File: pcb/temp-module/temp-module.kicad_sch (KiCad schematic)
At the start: 12 parts, among them J1 Connector_male, J2 Screw_Terminal_01x02, U1 MCP6002-xSN

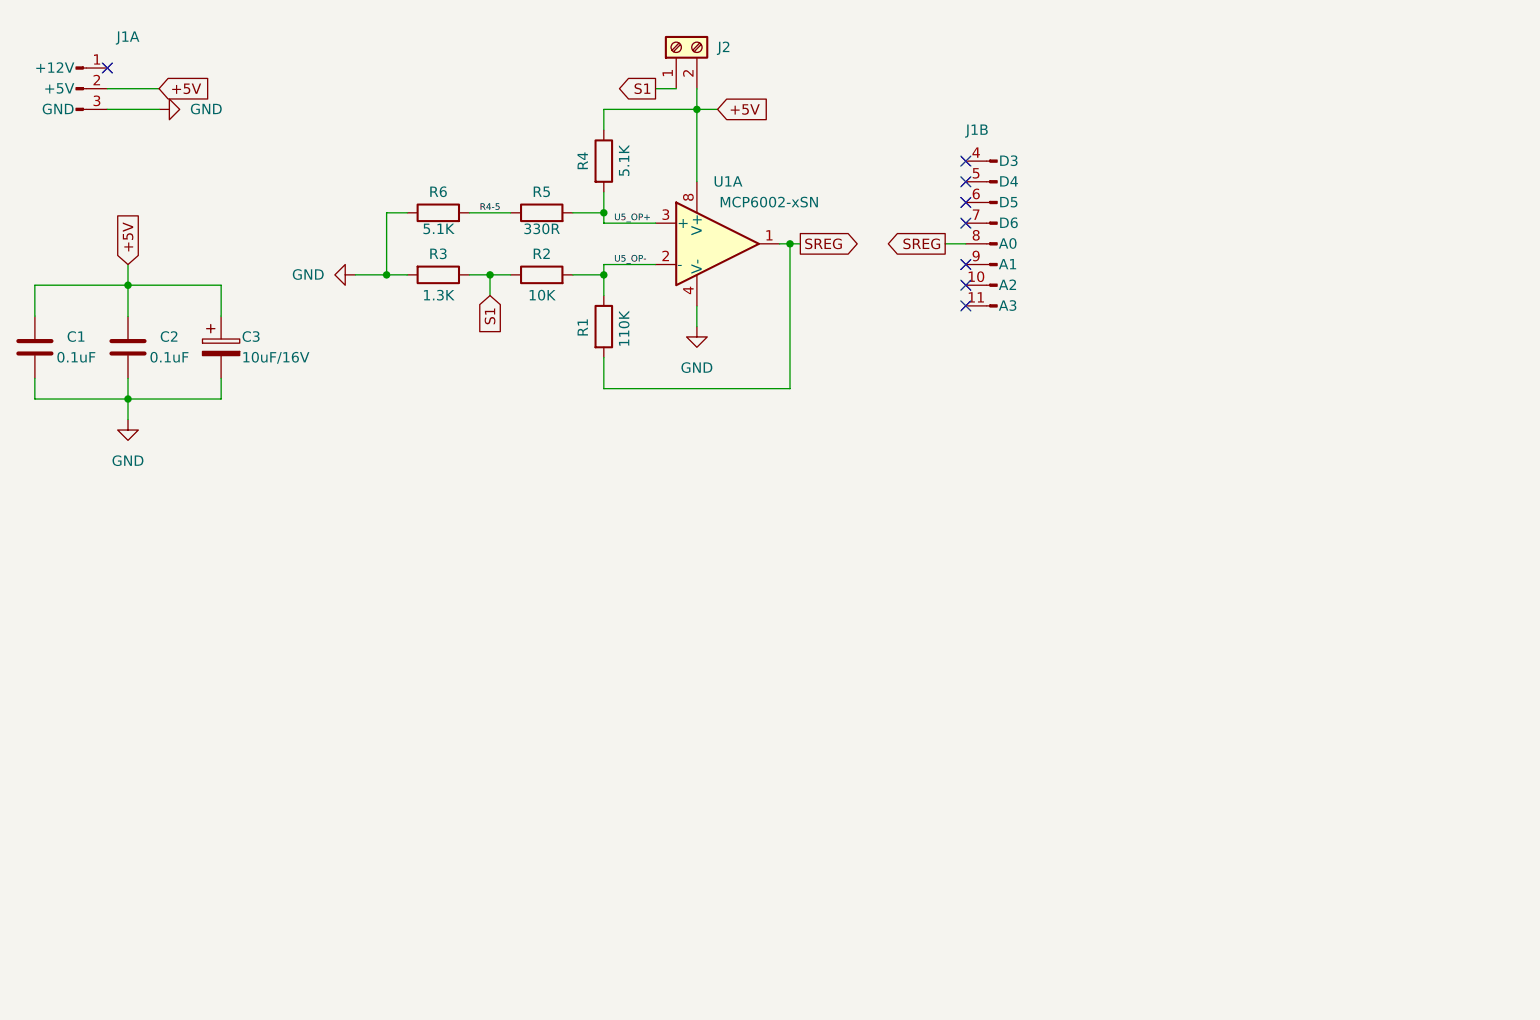
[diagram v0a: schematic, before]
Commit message: temp-calibrate
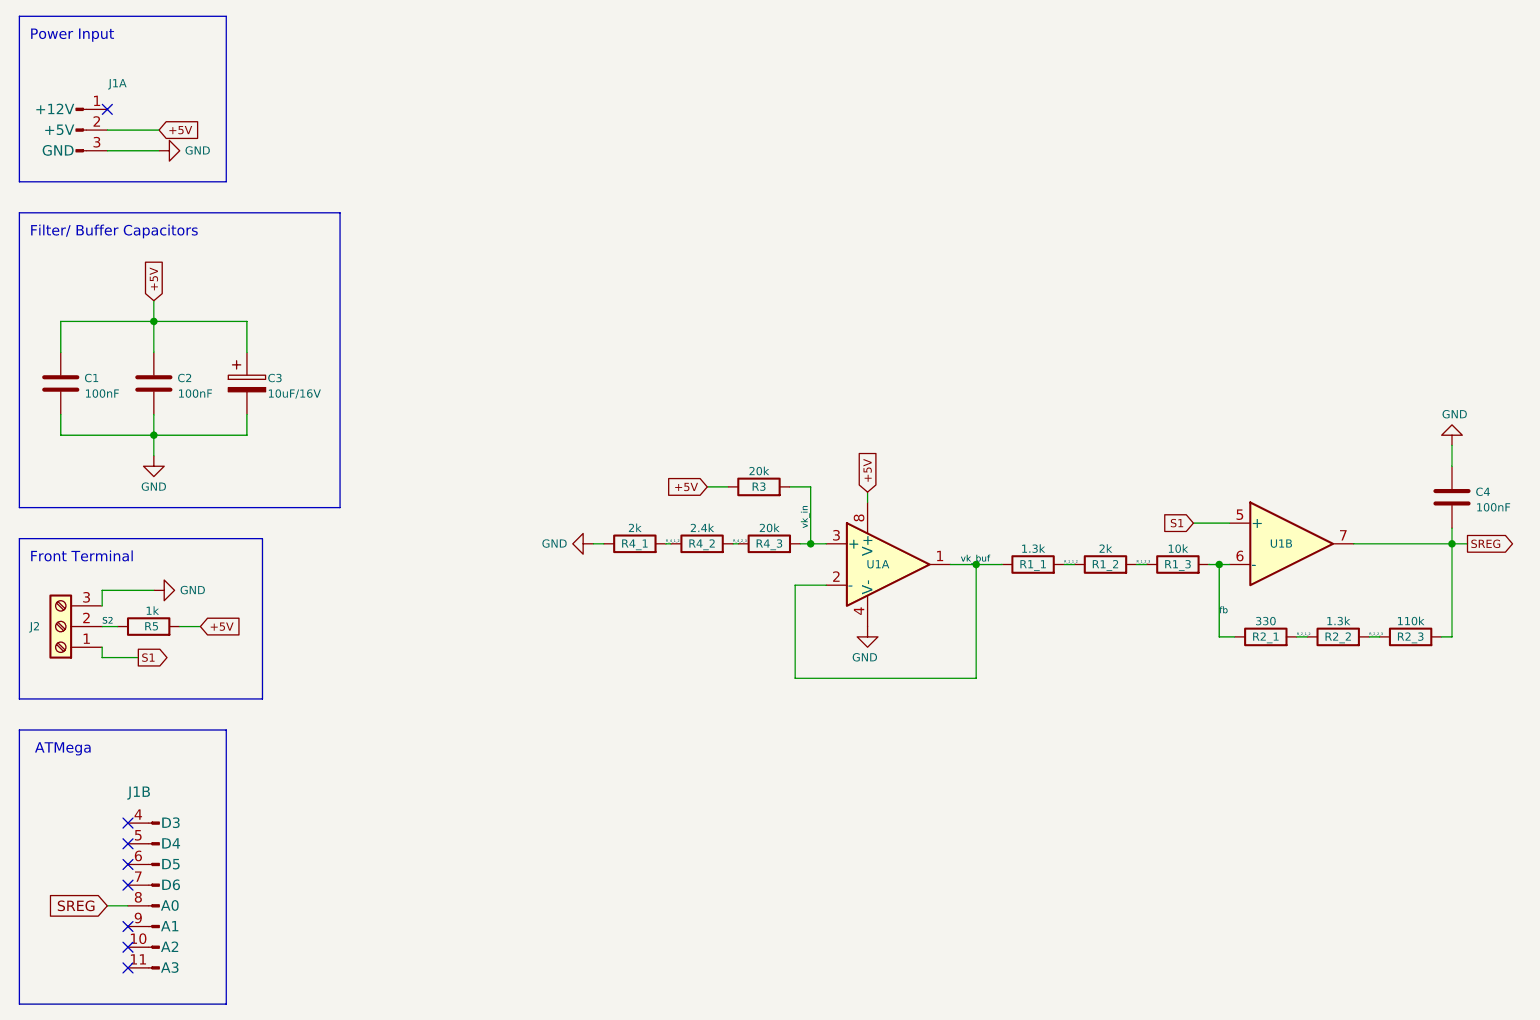
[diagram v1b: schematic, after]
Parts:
- removed J2: Screw_Terminal_01x02, TerminalBlock_Phoenix:TerminalBlock_Phoenix_MKDS-1,5-2-5.08_1x02_P5.08mm_Horizontal, symbol Connector:Screw_Terminal_01x02
- removed R1: 110K, Resistor_SMD:R_0805_2012Metric, symbol Device:R
- removed R2: 10K, Resistor_SMD:R_0805_2012Metric, symbol Device:R
- removed R4, R6: 5.1K, Resistor_SMD:R_0805_2012Metric, symbol Device:R
- removed U1: MCP6002-xSN, Package_DIP:DIP-8_W7.62mm, symbol Amplifier_Operational:MCP6002-xSN
- added C4: 100nF, Capacitor_SMD:C_1206_3216Metric, symbol Device:C
- added J2: Screw_Terminal_01x03, Connector_Wago:Wago_734-163_1x03_P3.50mm_Horizontal, symbol Connector:Screw_Terminal_01x03
- added R1_1, R2_2: 1.3k, Resistor_SMD:R_0805_2012Metric, symbol Device:R
- added R1_2, R4_1: 2k, Resistor_SMD:R_0805_2012Metric, symbol Device:R
- added R1_3: 10k, Resistor_SMD:R_0805_2012Metric, symbol Device:R
- added R2_1: 330, Resistor_SMD:R_0805_2012Metric, symbol Device:R
- added R2_3: 110k, Resistor_SMD:R_0805_2012Metric, symbol Device:R
- added R4_2: 2.4k, Resistor_SMD:R_0805_2012Metric, symbol Device:R
- added R4_3: 20k, Resistor_SMD:R_0805_2012Metric, symbol Device:R
- added U1: MCP6002-xP, Package_DIP:DIP-8_W7.62mm, symbol Amplifier_Operational:MCP6002-xP
- C1, C2: value 0.1uF -> 100nF
- R3: value 1.3K -> 20k
- R5: value 330R -> 1k
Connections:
- net U5_OP+ is gone; now on net +5V: R5.2
- net +5V: now also R3.1, U1.8 (V+)
- net GND: now also C4.1, J2.3 (Pin_3), R4_1.1, U1.4 (V-); no longer R3.2
- net S1: now also J2.1 (Pin_1), U1.5 (+); no longer R3.1
- net SREG: now also C4.2, R2_3.2, U1.7
- net R4-5 renamed S2
- net S2: now also J2.2 (Pin_2)
- new net R_1_1_2: R1_1.2, R1_2.1
- new net R_1_2_3: R1_2.2, R1_3.1
- new net R_2_1_2: R2_1.2, R2_2.1
- new net R_2_2_3: R2_2.2, R2_3.1
- new net R_4_1_2: R4_1.2, R4_2.1
- new net R_4_2_3: R4_2.2, R4_3.1
- new net fb: R1_3.2, R2_1.1, U1.6 (-)
- new net vk_buf: R1_1.1, U1.1, U1.2 (-)
- new net vk_in: R3.2, R4_3.2, U1.3 (+)
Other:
- note added: "ATMega"
- note added: "Filter/ Buffer Capacitors"
- note added: "Front Terminal"
- note added: "Power Input"
- moved on the sheet: C1, C2, C3, J1A, J1B
